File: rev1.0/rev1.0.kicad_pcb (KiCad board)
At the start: 2 copper layers, 39.4 x 27.9 mm, 14 parts, among them SW1 SW_DIP_x05, U1 74HC595, U2 74HC595, U3 74HC165

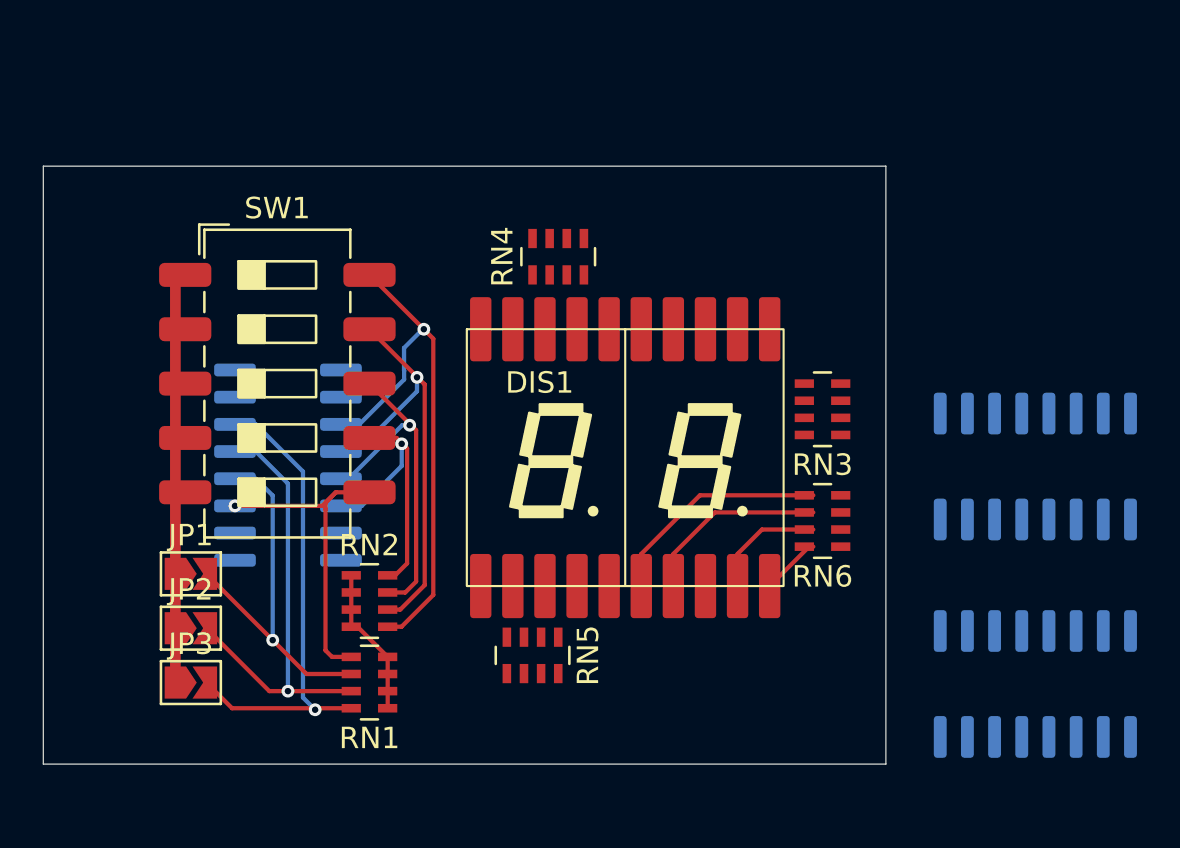
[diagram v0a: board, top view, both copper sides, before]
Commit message: More wokr. Må bare koble sammen headers og registere
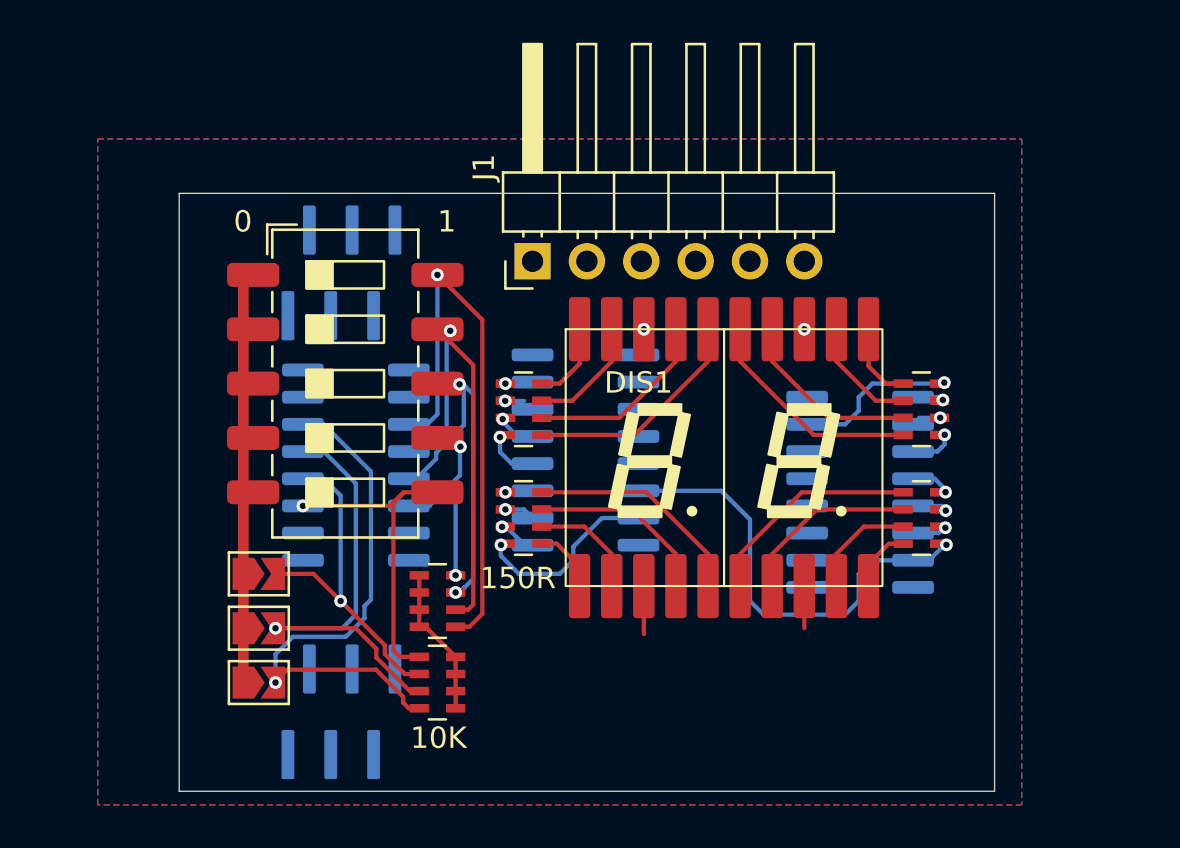
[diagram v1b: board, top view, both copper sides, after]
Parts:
- added J1: Conn_01x06_Pin, Connector_PinHeader_2.54mm:PinHeader_1x06_P2.54mm_Horizontal, F.Cu at (158.8, 89.5)
- added J3: Conn_01x06_Socket, timezoneClock:flatcable conn 6, B.Cu at (149.8, 90.1)
- added J4: Conn_01x06_Socket, timezoneClock:flatcable conn 6, B.Cu at (149.8, 110.6)
- moved U2 21.0 mm to (161.2, 98.4), turned to 0 degrees
- moved U1 12.1 mm to (174.1, 100.3), turned to 180 degrees
- moved RN4 7.31 mm to (158.3, 96.5), turned to 0 degrees
- moved RN5 6.43 mm to (158.3, 101.5), turned to 0 degrees
- moved RN6 4.62 mm to (176.9, 101.5)
- moved DIS1 4.62 mm to (167.7, 98.7)
- moved RN3 4.62 mm to (176.9, 96.5)
- moved JP1 3.18 mm to (146.0, 104.1)
- moved JP2 3.18 mm to (146.0, 106.7)
- moved JP3 3.18 mm to (146.0, 109.2)
- moved RN1 3.18 mm to (154.3, 109.2)
- moved RN2 3.18 mm to (154.3, 105.4)
- moved SW1 3.18 mm to (150.0, 95.2)
- moved U3 3.18 mm to (150.5, 99.1)
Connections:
- RN3 pad 1: unconnected-(RN3-R1.1-Pad1) -> Net-(RN3-R1.1)
- RN3 pad 2: unconnected-(RN3-R2.1-Pad2) -> Net-(RN3-R2.1)
- RN3 pad 3: unconnected-(RN3-R3.1-Pad3) -> Net-(RN3-R3.1)
- RN3 pad 4: unconnected-(RN3-R4.1-Pad4) -> Net-(RN3-R4.1)
- RN4 pad 1: unconnected-(RN4-R1.1-Pad1) -> Net-(RN4-R1.1)
- RN4 pad 2: unconnected-(RN4-R2.1-Pad2) -> Net-(RN4-R2.1)
- RN4 pad 3: unconnected-(RN4-R3.1-Pad3) -> Net-(RN4-R3.1)
- RN4 pad 4: unconnected-(RN4-R4.1-Pad4) -> Net-(RN4-R4.1)
- RN5 pad 1: unconnected-(RN5-R1.1-Pad1) -> Net-(RN5-R1.1)
- RN5 pad 2: unconnected-(RN5-R2.1-Pad2) -> Net-(RN5-R2.1)
- RN5 pad 3: unconnected-(RN5-R3.1-Pad3) -> Net-(RN5-R3.1)
- RN5 pad 4: unconnected-(RN5-R4.1-Pad4) -> Net-(RN5-R4.1)
- RN6 pad 1: unconnected-(RN6-R1.1-Pad1) -> Net-(RN6-R1.1)
- RN6 pad 2: unconnected-(RN6-R2.1-Pad2) -> Net-(RN6-R2.1)
- RN6 pad 3: unconnected-(RN6-R3.1-Pad3) -> Net-(RN6-R3.1)
- RN6 pad 4: unconnected-(RN6-R4.1-Pad4) -> Net-(RN6-R4.1)
- U1 pad 1: unconnected-(U1-QB-Pad1) -> Net-(RN3-R3.1)
- U1 pad 15: unconnected-(U1-QA-Pad15) -> Net-(RN3-R4.1)
- U1 pad 16: unconnected-(U1-VCC-Pad16) -> VCC
- U1 pad 2: unconnected-(U1-QC-Pad2) -> Net-(RN3-R2.1)
- U1 pad 3: unconnected-(U1-QD-Pad3) -> Net-(RN3-R1.1)
- U1 pad 4: unconnected-(U1-QE-Pad4) -> Net-(RN6-R4.1)
- U1 pad 5: unconnected-(U1-QF-Pad5) -> Net-(RN6-R3.1)
- U1 pad 6: unconnected-(U1-QG-Pad6) -> Net-(RN6-R2.1)
- U1 pad 7: Net-(U1-QH) -> Net-(RN6-R1.1)
- U1 pad 8: unconnected-(U1-GND-Pad8) -> GND
- U2 pad 1: unconnected-(U2-QB-Pad1) -> Net-(RN5-R3.1)
- U2 pad 14: Net-(U1-QH) -> Net-(RN6-R1.1)
- U2 pad 15: unconnected-(U2-QA-Pad15) -> Net-(RN5-R4.1)
- U2 pad 16: unconnected-(U2-VCC-Pad16) -> VCC
- U2 pad 2: unconnected-(U2-QC-Pad2) -> Net-(RN5-R2.1)
- U2 pad 3: unconnected-(U2-QD-Pad3) -> Net-(RN5-R1.1)
- U2 pad 4: unconnected-(U2-QE-Pad4) -> Net-(RN4-R4.1)
- U2 pad 5: unconnected-(U2-QF-Pad5) -> Net-(RN4-R3.1)
- U2 pad 6: unconnected-(U2-QG-Pad6) -> Net-(RN4-R2.1)
- U2 pad 7: unconnected-(U2-QH-Pad7) -> Net-(RN4-R1.1)
- U2 pad 8: unconnected-(U2-GND-Pad8) -> GND
- U3 pad 16: unconnected-(U3-VCC-Pad16) -> VCC
- U3 pad 8: unconnected-(U3-GND-Pad8) -> GND
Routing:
- net Net-(RN6-R1.1): track 0.00 -> 21.1 mm, vias 0 -> 1
- net Net-(RN4-R4.2): track 0.00 -> 10.7 mm
- net Net-(RN3-R1.2): track 0.00 -> 10.5 mm
- net Net-(RN5-R1.2): track 0.00 -> 10.5 mm
- net Net-(RN4-R3.2): track 0.00 -> 8.86 mm
- net Net-(RN5-R4.1): track 0.00 -> 8.76 mm, vias 0 -> 1
- net Net-(RN3-R2.2): track 0.00 -> 8.71 mm
- net Net-(RN5-R2.2): track 0.00 -> 8.63 mm
- net Net-(RN3-R4.1): track 0.00 -> 7.59 mm, vias 0 -> 1
- net Net-(RN4-R2.2): track 0.00 -> 5.53 mm
- net Net-(RN3-R3.2): track 0.00 -> 5.38 mm
- net Net-(RN5-R3.2): track 0.00 -> 5.30 mm
- net GND: track 7.08 -> 11.3 mm, vias 0 -> 2
- net Net-(RN4-R1.2): track 0.00 -> 3.77 mm
- net Net-(RN3-R4.2): track 0.00 -> 3.69 mm
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- added copper zone on B.Cu, net GND
- added copper zone on F.Cu, net GND
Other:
- board size 39.4 x 27.9 mm -> 38.1 x 27.9 mm
- board text added: "0"
- board text added: "1"
- board text added: "10K"
- board text added: "150R"
